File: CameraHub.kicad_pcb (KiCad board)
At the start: 4 copper layers, 95.9 x 90.2 mm, 122 parts, among them J1 200528-0120, J10 Header 01x04 0.1", J11 Header 01x04 0.1", J2 Conn_01x02, J3 Conn_01x02, J4 USB_C_Receptacle_USB2.0_16P, J5 USB_C_Receptacle_USB2.0_16P, J6 Header 01x04 0.1", J7 USB_C_Receptacle_USB2.0_16P, J8 USB_C_Receptacle_USB2.0_16P, J9 Header 01x04 0.1", U1 USBLC6-2P6, U10 USB2514B-I/M2, U11 MIC2026-1xM, U12 MIC2026-1xM, U14 TLV76733QWDRBxQ1, U2 USBLC6-2P6, U3 USBLC6-2P6, U4 USB2514B-I/M2, U5 MIC2026-1xM, U6 MIC2026-1xM, U7 USBLC6-2P6, U8 USBLC6-2P6, U9 USBLC6-2P6, Y1 24MHz, Y2 24MHz

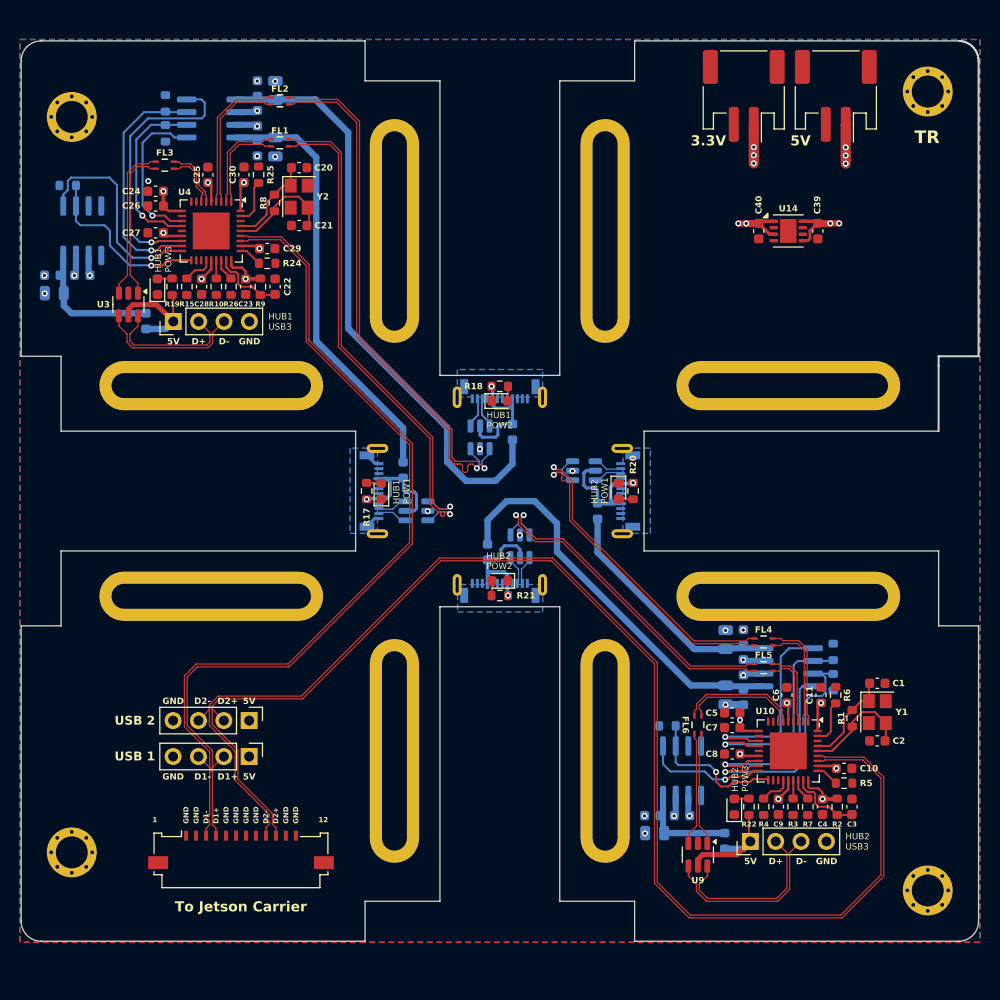
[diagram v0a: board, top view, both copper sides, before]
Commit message: Complete layout
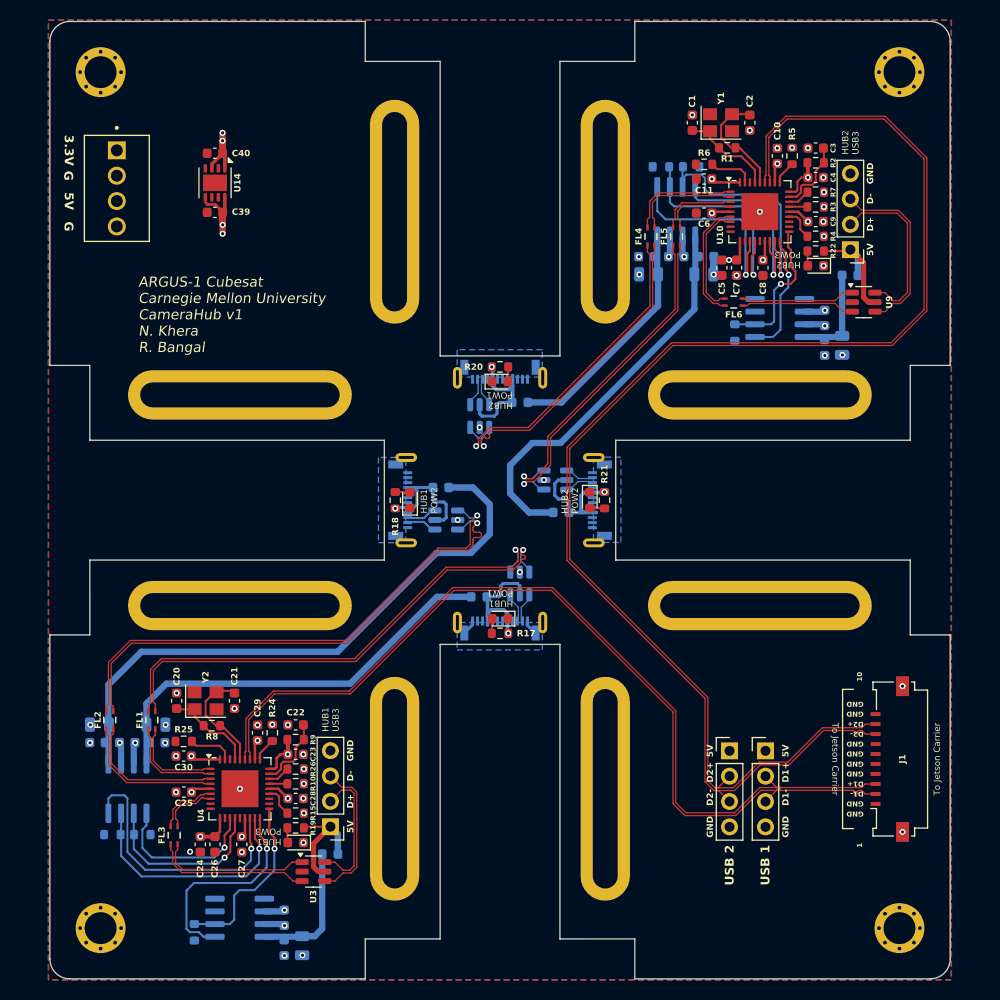
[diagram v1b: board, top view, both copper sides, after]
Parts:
- removed the J2 at (173.3, 56.3)
- removed the J3 at (182.5, 56.3)
- added J10: TE_282834-4, CameraHub:TE_282834-4, F.Cu at (110.5, 65.6)
- J1: value 200528-0120 -> 200528-0100; footprint Connector_FFC-FPC:Molex_200528-0120_1x12-1MP_P1.00mm_Horizontal -> Connector_FFC-FPC:Molex_200528-0100_1x10-1MP_P1.00mm_Horizontal
- moved H3 83.2 mm to (188.9, 139.7), turned to -90 degrees
- moved H1 82.9 mm to (108.9, 54.0), turned to -90 degrees
- moved H4 82.0 mm to (188.9, 54.0), turned to -90 degrees
- moved H2 81.3 mm to (108.9, 139.7), turned to -90 degrees
- moved R33 75.9 mm to (118.3, 140.1), turned to 90 degrees
- moved R31 73.4 mm to (110.1, 130.3), turned to 0 degrees
- moved C38 71.2 mm to (127.3, 141.7), turned to -90 degrees
- moved U6 70.6 mm to (122.8, 138.7), turned to 0 degrees
- moved R30 70.3 mm to (113.1, 130.3), turned to 180 degrees
- moved C37 69.9 mm to (129.1, 141.5), turned to -90 degrees
- moved U5 67.6 mm to (111.6, 125.7), turned to 90 degrees
- moved C36 67.5 mm to (127.3, 138.7), turned to 90 degrees
- moved C33 67.4 mm to (108.6, 121.1), turned to 180 degrees
- moved FL3 67.1 mm to (116.3, 130.4), turned to -90 degrees
- moved C3 66.1 mm to (180.5, 61.6), turned to 180 degrees
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- renumbered J10 to J2, J11 to J3
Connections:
- J1 pad 10: /USB2_P -> GND
- J1 pad 2: GND -> /USB1_N
- J1 pad 3: /USB1_N -> /USB1_P
- J1 pad 4: /USB1_P -> GND
- J1 pad 8: GND -> /USB2_N
- J1 pad 9: /USB2_N -> /USB2_P
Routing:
- net +5V: track 19.5 -> 15.0 mm, vias 9 -> 6
- net +3.3V: track 48.5 -> 44.6 mm, vias 19 -> 16
- net /USB1_P: track 88.0 -> 91.1 mm
- net /USB1_N: track 87.9 -> 91.0 mm
- net /USB2_P: track 137.5 -> 140.6 mm
- net /USB2_N: track 138.3 -> 141.2 mm
- net GND: vias 20 -> 50
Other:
- board size 95.9 x 90.2 mm -> 90.2 x 95.9 mm
- board text added: "10"
- board text added: "G"
- board text removed: "12"
- board text removed: "TR"
